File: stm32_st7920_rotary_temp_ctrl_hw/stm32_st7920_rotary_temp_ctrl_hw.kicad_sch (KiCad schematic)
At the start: 145 parts, among them IC1 MAX6675, J1 USB_C_Receptacle_USB2.0, J2 CONN_01X04, Q1 C1815, Q10 C1815, Q11 C1815, Q12 C1815, Q13 IRF3205, Q2 C1815, Q3 C1815, Q4 C1815, Q5 ME15N10, Q6 C1815, Q7 C1815, Q8 IRF3205, Q9 C1815, SW1 RotaryEncoder_Switch, SW2 BT_1, SW3 BT_1, U1 XL1509, U2 74HC245, U3 STM32F103C8, U4 ASM1117, U5 MAX485, Y1 8MHz, Y2 32,768KHz

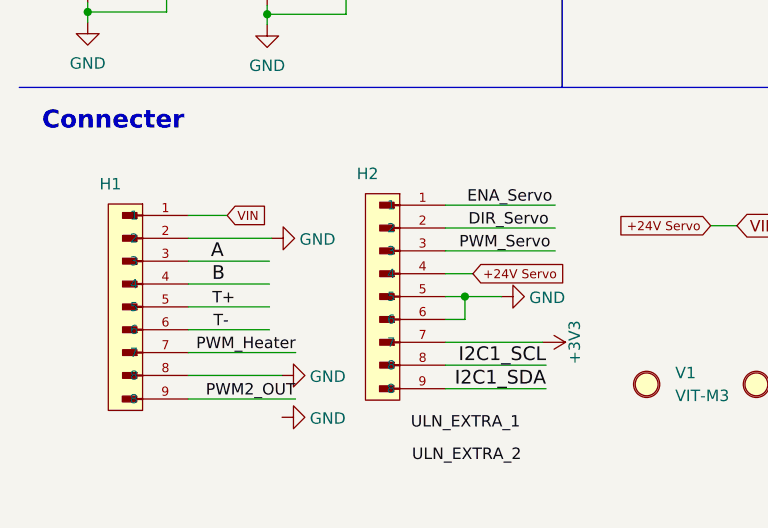
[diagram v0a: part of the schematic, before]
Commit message: Start layout
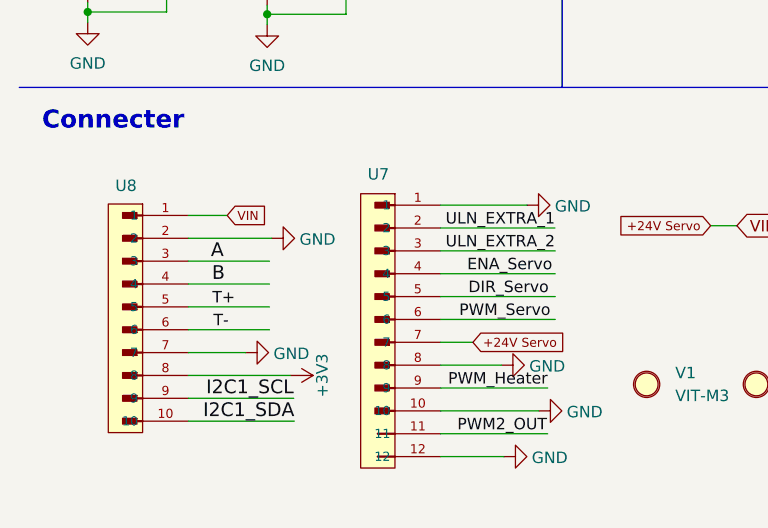
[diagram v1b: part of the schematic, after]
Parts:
- removed H1, H2: ~, Lib_Hien:KF142_9P_5.08, symbol Lib_Hien:KF142-5.08-9P
- added U7: ~, Lib_Hien:KF142_12P_5.08, symbol Lib_Hien:XH-12P-2.54
- added U8: ~, Lib_Hien:KF142_10P_5.08, symbol Lib_Hien:XH-10P-2.54
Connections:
- net +24V Servo: now also U7.7, U8.1
- net +3V3: now also U8.8
- net A: now also U8.3
- net B: now also U8.4
- net DIR_Servo: now also U7.5
- net ENA_Servo: now also U7.4
- net GND: now also U7.1, U7.10, U7.12, U7.8, U8.2, U8.6, U8.7
- net I2C1_SCL: now also U8.9
- net I2C1_SDA: now also U8.10
- net PWM2_OUT: now also U7.11
- net PWM_Heater: now also U7.9
- net PWM_Servo: now also U7.6
- net T+: now also U8.5
- net ULN_EXTRA_1: now also U7.2
- net ULN_EXTRA_2: now also U7.3
